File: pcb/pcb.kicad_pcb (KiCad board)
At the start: 2 copper layers, 99.1 x 90.2 mm, 68 parts, among them J1 Conn_01x01, J2 Conn_01x01, J3 Conn_01x01, SW1 SW_PUSH, SW2 SW_PUSH, SW3 SW_PUSH, SW4 SW_PUSH, SW5 SW_PUSH, SW6 SW_PUSH, SW7 SW_PUSH, SW8 SW_PUSH, SW9 SW_PUSH, U1 ProMicro

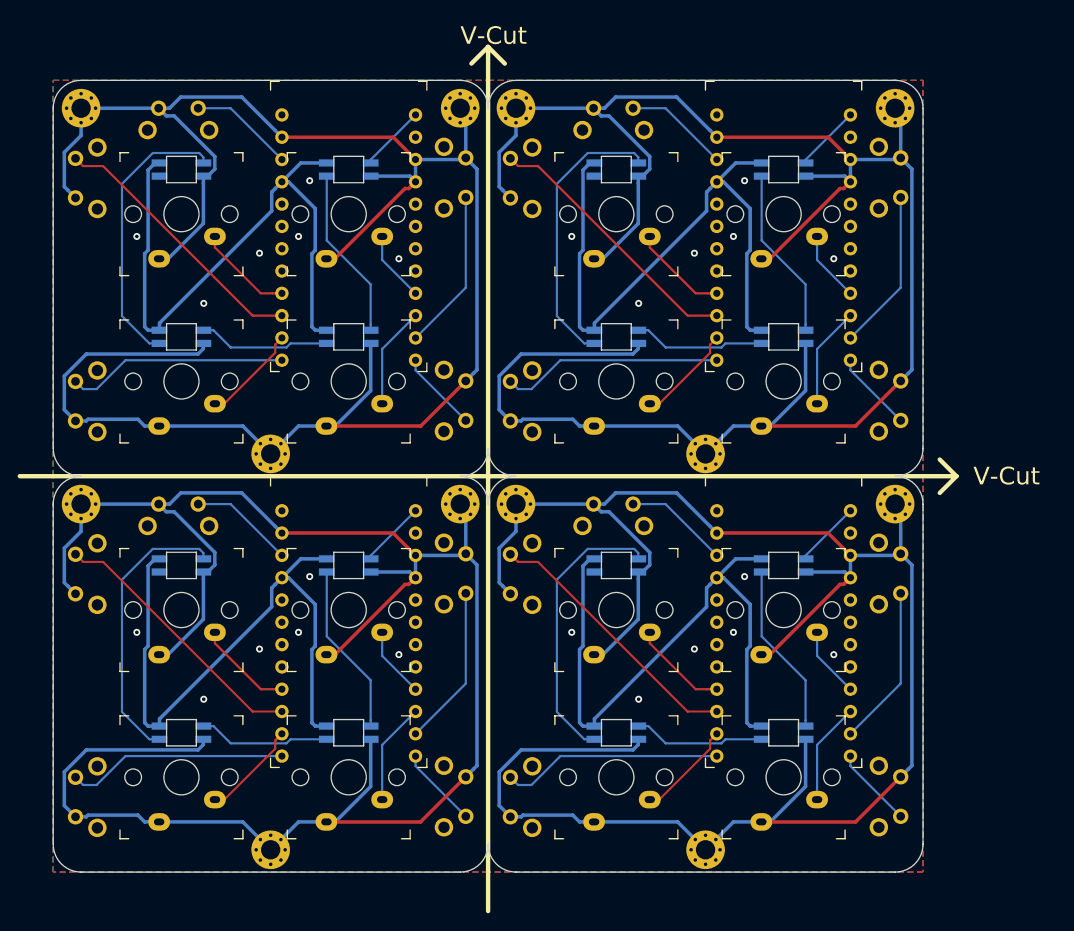
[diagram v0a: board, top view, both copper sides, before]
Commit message: create rubykaigi 2023
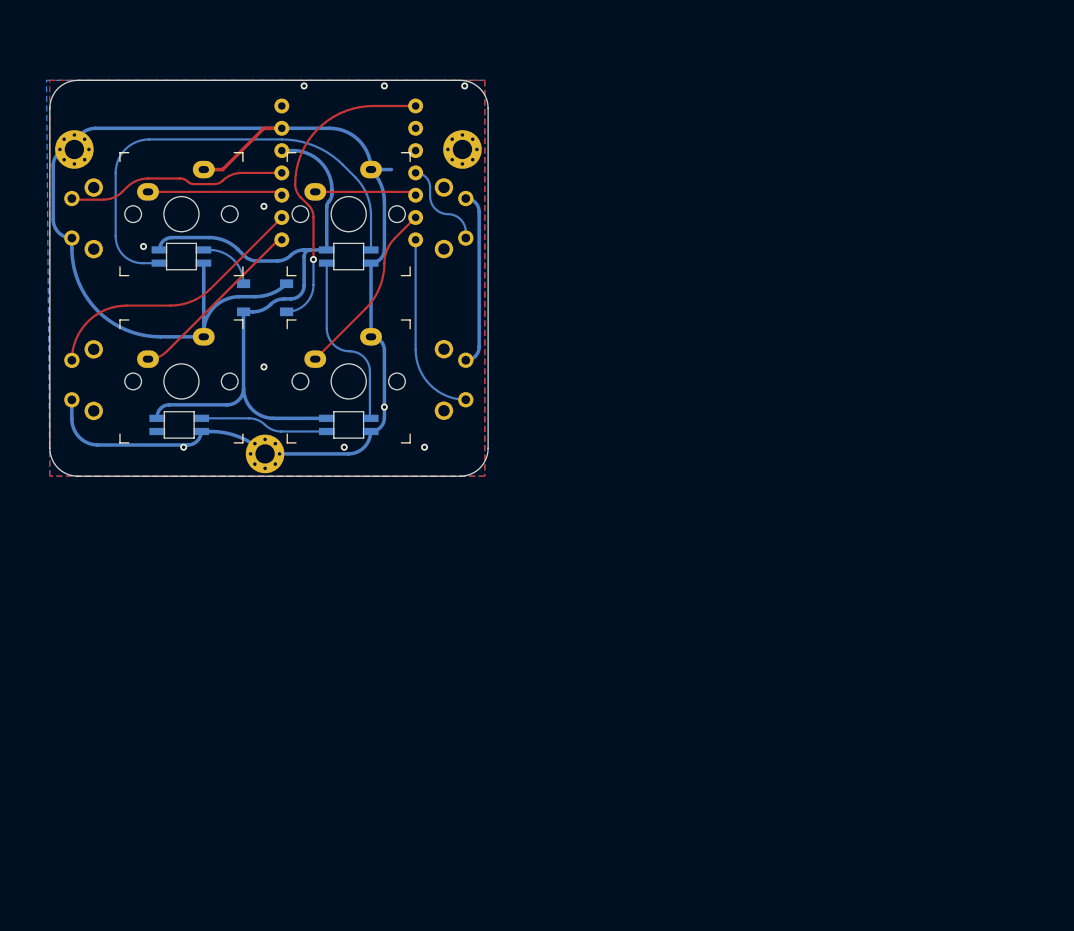
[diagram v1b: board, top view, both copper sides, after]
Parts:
- removed the J1 at (115.6, 98.4)
- removed the J1 at (66.0, 98.4)
- removed the J1 at (115.6, 53.3)
- removed the J2 at (137.2, 137.8)
- removed the J2 at (87.6, 137.8)
- removed the J2 at (137.2, 92.7)
- removed the J3 at (158.8, 98.4)
- removed the J3 at (109.2, 98.4)
- removed the J3 at (158.8, 53.3)
- removed the L1 at (146.1, 105.4)
- removed the L1 at (96.5, 105.4)
- removed the L1 at (146.1, 60.3)
- removed the L2 at (146.1, 124.5)
- removed the L2 at (96.5, 124.5)
- removed the L2 at (146.1, 79.4)
- removed the L3 at (127.0, 124.5)
- removed the L3 at (77.5, 124.5)
- removed the L3 at (127.0, 79.4)
- removed the L4 at (127.0, 105.4)
- removed the L4 at (77.5, 105.4)
- removed the L4 at (127.0, 60.3)
- removed the SW1 at (146.1, 110.5)
- removed the SW1 at (96.5, 110.5)
- removed the SW1 at (146.1, 65.4)
- removed the SW2 at (146.1, 129.5)
- removed the SW2 at (96.5, 129.5)
- removed the SW2 at (146.1, 84.5)
- removed the SW3 at (159.4, 108.6)
- removed the SW3 at (109.9, 108.6)
- removed the SW3 at (159.4, 63.5)
- removed the SW4 at (159.4, 134.0)
- removed the SW4 at (109.9, 134.0)
- removed the SW4 at (159.4, 88.9)
- removed the SW5 at (127.0, 110.5)
- removed the SW5 at (77.5, 110.5)
- removed the SW5 at (127.0, 65.4)
- removed the SW6 at (127.0, 129.5)
- removed the SW6 at (77.5, 129.5)
- removed the SW6 at (127.0, 84.5)
- removed the SW7 at (114.9, 104.1)
- removed the SW7 at (65.4, 104.1)
- removed the SW7 at (114.9, 59.1)
- removed the SW8 at (114.9, 129.5)
- removed the SW8 at (65.4, 129.5)
- removed the SW8 at (114.9, 84.5)
- removed SW9 (x4): SW_PUSH, Button_Switch_THT:SW_Tactile_SPST_Angled_PTS645Vx39-2LFS
- removed the U1 at (96.5, 113.7)
- removed the U1 at (146.1, 113.7)
- removed the U1 at (146.1, 68.6)
- removed the U1 at (96.5, 68.6)
- added L5: YS-SK6812MINI, Keyboard:YS-SK6812MINI-E, B.Cu at (77.2, 89.4)
- added U1: SeeeduinoXIAO, Keyboard:Seeeduino XIAO TH only, B.Cu at (96.5, 60.7)
- L1: footprint Keyboard:YS-SK6812MINI-E -> LED_SMD:LED_WS2812B_PLCC4_5.0x5.0mm_P3.2mm
- SW1, SW5: footprint Keyboard:MX_1U -> Button_Switch_THT:SW_Tactile_SPST_Angled_PTS645Vx39-2LFS; moved to B.Cu
- SW3, SW7: footprint Button_Switch_THT:SW_Tactile_SPST_Angled_PTS645Vx39-2LFS -> Keyboard:MX_1U; moved to F.Cu
- moved SW8 44.5 mm to (109.9, 86.5), turned to 90 degrees
- moved SW7 40.2 mm to (96.5, 84.5), turned to 0 degrees
- moved L4 34.8 mm to (96.5, 89.4)
- moved SW1 31.6 mm to (65.0, 63.6), turned to -90 degrees
- moved SW2 26.9 mm to (77.5, 65.4), turned to 0 degrees
- moved L2 21.1 mm to (77.5, 70.2)
- moved L3 21.1 mm to (96.5, 70.2)
- moved SW5 20.8 mm to (65.0, 82.1), turned to -90 degrees
- moved SW4 20.8 mm to (109.9, 68.1)
- moved L1 17.4 mm to (87.0, 74.9), turned to 0 degrees
- moved SW3 13.5 mm to (96.5, 65.4), turned to 0 degrees
- moved J1 4.76 mm to (65.3, 58.0)
- moved J3 4.71 mm to (109.5, 58.0)
- moved J2 0.63 mm to (87.0, 92.7)
- turned SW6 to 0 degrees
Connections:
- L4 pad 2: (no net) -> Net-(L4-Pad2)
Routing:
- net GND: track 888.5 -> 211.1 mm, vias 24 -> 10
- net VCC: track 282.8 -> 80.3 mm
- net Net-(L3-Pad2): track 128.8 -> 20.3 mm
- net SW7: track 123.7 -> 20.3 mm
- net SW8: track 100.9 -> 21.2 mm
- net Net-(L1-Pad2): track 78.5 -> 6.62 mm
- net SW3: track 76.0 -> 11.6 mm
- net RESET: track 47.8 -> 0.00 mm
- net SW2: track 46.4 -> 15.4 mm
- net SW4: track 36.9 -> 10.5 mm
- net SW6: track 45.1 -> 20.7 mm
- net Net-(L4-Pad2): track 0.00 -> 14.7 mm
- net SW5: track 44.2 -> 31.1 mm
- net SW1: track 32.2 -> 25.1 mm
- net Net-(L2-Pad2): track 60.2 -> 53.2 mm
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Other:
- board size 99.1 x 90.2 mm -> 49.9 x 45.1 mm
- net class Default removed
- net class PWR removed
- board text added: "Matsumoto Performing Arts Centre May 11th - 13th"
- board text added: "PCB Designed by @swan_match"
- board text added: "RubyKaigi 2023"
- board text removed: "Designed by @swan_match"
- board text removed: "SouthernCross"
- board text removed: "V-Cut"
